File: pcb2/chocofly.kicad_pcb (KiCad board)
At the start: 2 copper layers, 341.3 x 148.9 mm, 173 parts, among them P1 battery+, P2 battery-, SW1 SW_Push, SW11 SW_Push, SW12 SW_Push, SW13 SW_Push, SW14 SW_Push, SW15 SW_Push, SW16 SW_Push, SW17 SW_Push, SW18 SW_Push, SW19 SW_Push, SW2 SW_Push, SW20 SW_Push, SW21 SW_Push, SW22 SW_Push, SW23 SW_Push, SW24 SW_Push, SW25 SW_Push, SW26 SW_Push, SW27 SW_Push, SW28 SW_Push, SW29 SW_Push, SW3 SW_Push, SW30 SW_Push, SW31 SW_Push, SW32 SW_Push, SW33 SW_Push, SW34 SW_Push, SW35 SW_Push, SW36 SW_Push, SW37 SW_Push, SW38 SW_Push, SW39 SW_Push, SW4 SW_Push, SW40 SW_Push, SW41 SW_Push, SW42 SW_Push, SW43 SW_Push, SW44 SW_Push, SW45 SW_Push, SW46 SW_Push, SW47 SW_Push, SW48 SW_Push, SW49 SW_Push, SW5 SW_Push, SW50 SW_Push, SW51 SW_Push, SW52 SW_Push, SW53 SW_Push, SW54 SW_Push, SW55 SW_Push, SW56 SW_Push, SW57 SW_Push, SW58 SW_Push, SW59 SW_Push, SW6 SW_Push, SW60 SW_Push, SW61 SW_Push, SW62 Reset, SW63 Power, SW7 SW_Push, SW8 SW_Push, SW9 SW_Push

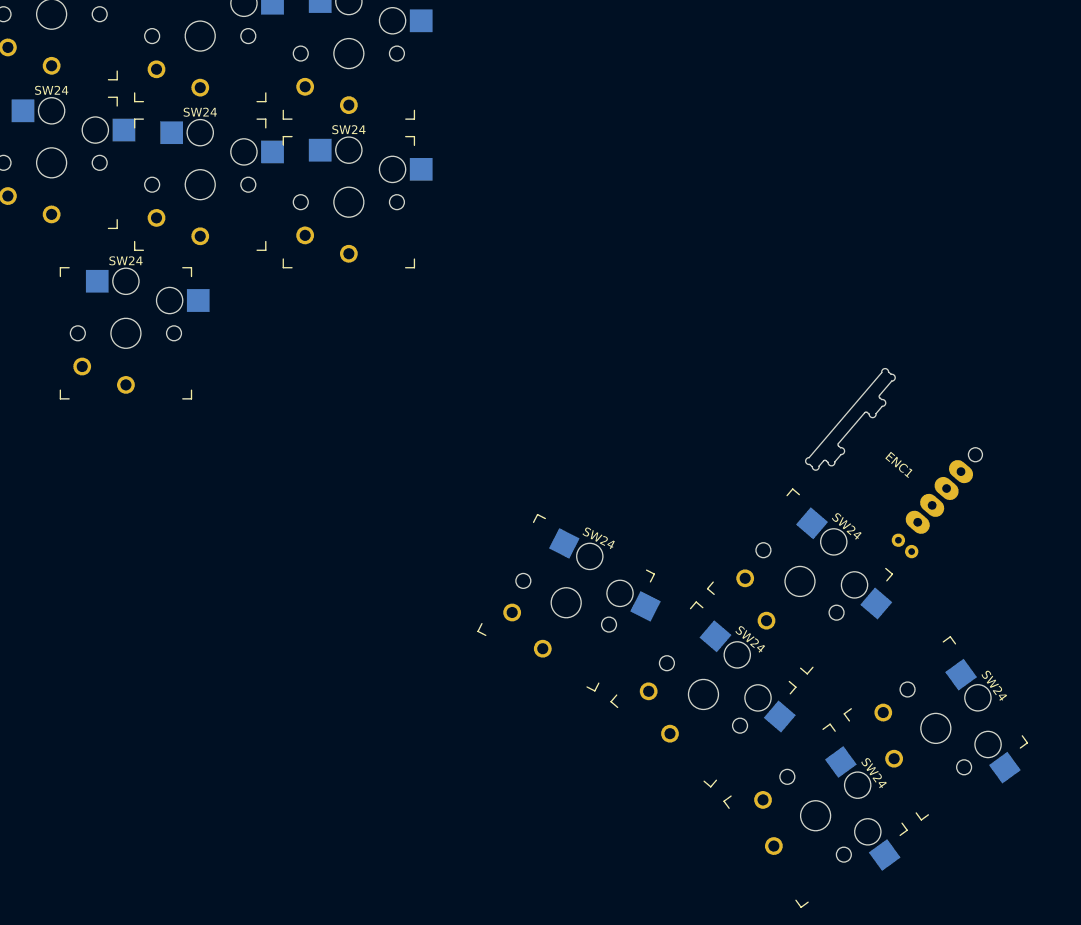
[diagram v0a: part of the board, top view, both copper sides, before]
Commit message: wip
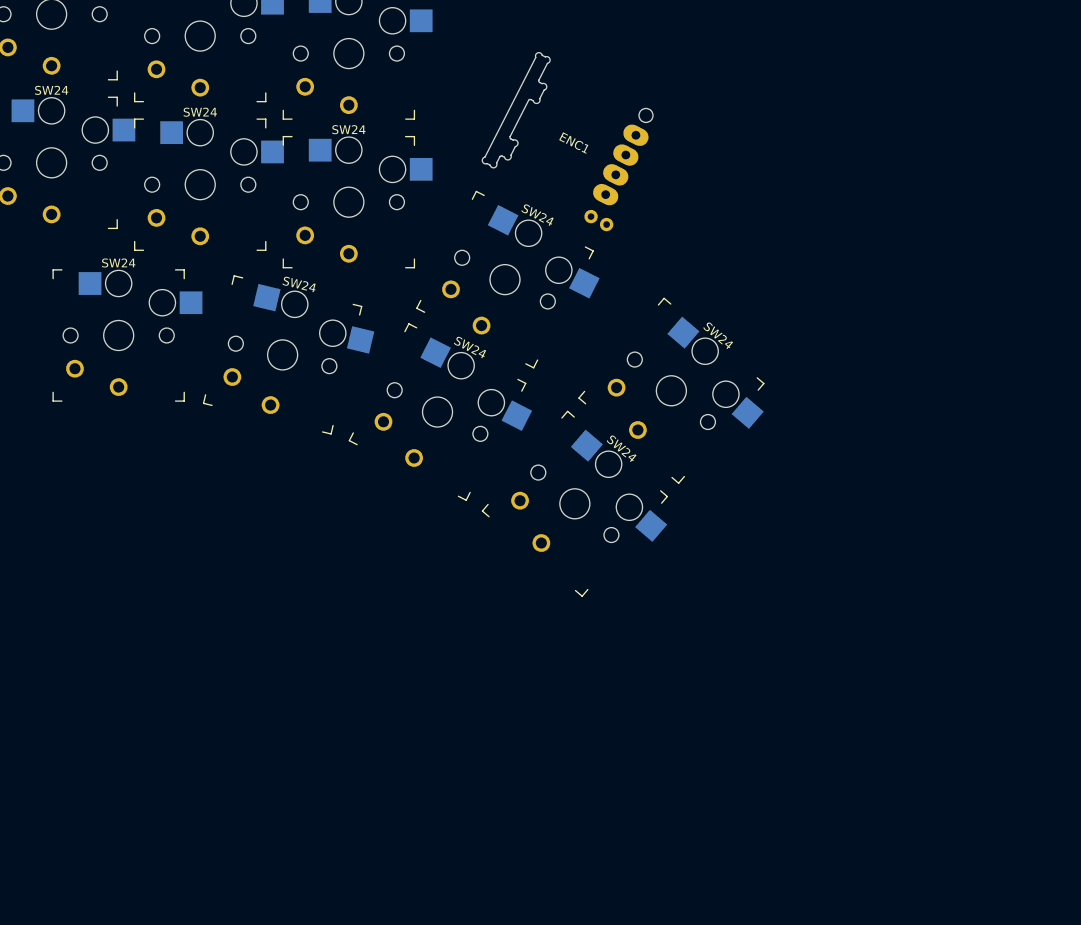
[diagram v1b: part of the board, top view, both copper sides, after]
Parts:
- removed the SW24 at (22.1, 243.2)
- removed the SW24 at (6.60, 226.4)
- removed the SW24 at (8.39, 253.2)
- removed the SW24 at (-4.44, 239.3)
- added SW24: SW_Push, footprints:Kailh_socket_PG1350_optional_chosfox, F.Cu at (-8.11, 204.6)
- added SW24: SW_Push, footprints:Kailh_socket_PG1350_optional_chosfox, F.Cu at (-27.1, 191.9)
- added SW24: SW_Push, footprints:Kailh_socket_PG1350_optional_chosfox, F.Cu at (-19.1, 217.5)
- added SW24: SW_Push, footprints:Kailh_socket_PG1350_optional_chosfox, F.Cu at (-34.9, 207.0)
- moved ENC1 52.3 mm to (-19.2, 176.3), turned to 153 degrees
- moved SW24 43.1 mm to (-52.6, 200.5), turned to 346.5 degrees
- moved SW24 0.87 mm to (-71.3, 198.2)

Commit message: General layout is ready
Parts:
- removed the ENC1 at (-19.2, 176.3)
- removed the SW24 at (-8.11, 204.6)
- removed the SW24 at (-131.4, 168.5)
- removed the SW24 at (-45.0, 166.0)
- removed the SW24 at (-62.0, 181.0)
- removed the SW24 at (-96.0, 164.0)
- removed the SW24 at (-130.3, 185.5)
- removed the SW24 at (-96.0, 181.0)
- removed the SW24 at (-114.4, 167.5)
- removed the SW24 at (-79.0, 178.5)
- removed the SW24 at (-113.4, 184.4)
- removed the SW24 at (-45.0, 183.0)
- removed the SW24 at (-27.1, 191.9)
- removed the SW24 at (-79.0, 144.5)
- removed the SW24 at (-62.0, 147.0)
- removed the SW24 at (-132.4, 151.5)
- removed the SW24 at (-45.0, 149.0)
- removed the SW24 at (-96.0, 147.0)
- removed the SW24 at (-115.4, 150.5)
- removed the SW24 at (-45.0, 132.0)
- removed the SW24 at (-62.0, 130.0)
- removed the SW24 at (-79.0, 127.5)
- removed the SW24 at (-96.0, 130.0)
- removed the SW24 at (-19.1, 217.5)
- removed the SW24 at (-116.5, 133.5)
- removed the SW24 at (-34.9, 207.0)
- removed the SW24 at (-52.6, 200.5)
- removed the SW24 at (-71.3, 198.2)
- removed the SW24 at (-133.4, 134.6)
- removed the SW24 at (-79.0, 161.5)
- removed the SW24 at (-62.0, 164.0)
- added ENC1: EVQWGD001, footprints:EVQWGD001, F.Cu at (-15.3, 219.8)
- added ENC1: EVQWGD001, footprints:EVQWGD001, F.Cu at (-53.7, 219.8)
- added SW24: SW_Push, footprints:Kailh_socket_PG1350_optional_chosfox, F.Cu at (-19.5, 249.9)
- added SW24: SW_Push, footprints:Kailh_socket_PG1350_optional_chosfox, F.Cu at (72.2, 172.3)
- added SW24: SW_Push, footprints:Kailh_socket_PG1350_optional_chosfox, F.Cu at (52.5, 173.4)
- added SW24: SW_Push, footprints:Kailh_socket_PG1350_optional_chosfox, F.Cu at (56.5, 190.0)
- added SW24: SW_Push, footprints:Kailh_socket_PG1350_optional_chosfox, F.Cu at (27.4, 214.4)
- added SW24: SW_Push, footprints:Kailh_socket_PG1350_optional_chosfox, F.Cu at (91.9, 186.1)
- added SW24: SW_Push, footprints:Kailh_socket_PG1350_optional_chosfox, F.Cu at (75.2, 189.0)
- added SW24: SW_Push, footprints:Kailh_socket_PG1350_optional_chosfox, F.Cu at (94.9, 202.8)
- added SW24: SW_Push, footprints:Kailh_socket_PG1350_optional_chosfox, F.Cu at (39.4, 191.5)
- added SW24: SW_Push, footprints:Kailh_socket_PG1350_optional_chosfox, F.Cu at (7.36, 203.8)
- added SW24: SW_Push, footprints:Kailh_socket_PG1350_optional_chosfox, F.Cu at (86.0, 152.6)
- added SW24: SW_Push, footprints:Kailh_socket_PG1350_optional_chosfox, F.Cu at (40.5, 229.0)
- added SW24: SW_Push, footprints:Kailh_socket_PG1350_optional_chosfox, F.Cu at (89.0, 169.4)
- added SW24: SW_Push, footprints:Kailh_socket_PG1350_optional_chosfox, F.Cu at (3.39, 187.3)
- added SW24: SW_Push, footprints:Kailh_socket_PG1350_optional_chosfox, F.Cu at (23.4, 197.9)
- added SW24: SW_Push, footprints:Kailh_socket_PG1350_optional_chosfox, F.Cu at (78.1, 205.8)
- added SW24: SW_Push, footprints:Kailh_socket_PG1350_optional_chosfox, F.Cu at (15.5, 164.9)
- added SW24: SW_Push, footprints:Kailh_socket_PG1350_optional_chosfox, F.Cu at (-0.58, 170.8)
- added SW24: SW_Push, footprints:Kailh_socket_PG1350_optional_chosfox, F.Cu at (48.5, 156.9)
- added SW24: SW_Push, footprints:Kailh_socket_PG1350_optional_chosfox, F.Cu at (43.3, 208.0)
- added SW24: SW_Push, footprints:Kailh_socket_PG1350_optional_chosfox, F.Cu at (35.4, 175.0)
- added SW24: SW_Push, footprints:Kailh_socket_PG1350_optional_chosfox, F.Cu at (11.3, 220.4)
- added SW24: SW_Push, footprints:Kailh_socket_PG1350_optional_chosfox, F.Cu at (69.3, 155.6)
- added SW24: SW_Push, footprints:Kailh_socket_PG1350_optional_chosfox, F.Cu at (60.5, 206.5)
- added SW24: SW_Push, footprints:Kailh_socket_PG1350_optional_chosfox, F.Cu at (-49.6, 249.9)
- added SW24: SW_Push, footprints:Kailh_socket_PG1350_optional_chosfox, F.Cu at (-65.1, 233.1)
- added SW24: SW_Push, footprints:Kailh_socket_PG1350_optional_chosfox, F.Cu at (-63.3, 259.9)
- added SW24: SW_Push, footprints:Kailh_socket_PG1350_optional_chosfox, F.Cu at (-76.1, 246.1)
- added SW24: SW_Push, footprints:Kailh_socket_PG1350_optional_chosfox, F.Cu at (-91.8, 235.6)
- added SW24: SW_Push, footprints:Kailh_socket_PG1350_optional_chosfox, F.Cu at (-109.6, 229.0)
- added SW24: SW_Push, footprints:Kailh_socket_PG1350_optional_chosfox, F.Cu at (-155.1, 152.6)
- added SW24: SW_Push, footprints:Kailh_socket_PG1350_optional_chosfox, F.Cu at (-108.4, 191.5)
- added SW24: SW_Push, footprints:Kailh_socket_PG1350_optional_chosfox, F.Cu at (-92.5, 197.9)
- added SW24: SW_Push, footprints:Kailh_socket_PG1350_optional_chosfox, F.Cu at (22.8, 235.6)
- added SW24: SW_Push, footprints:Kailh_socket_PG1350_optional_chosfox, F.Cu at (-161.0, 186.1)
- added SW24: SW_Push, footprints:Kailh_socket_PG1350_optional_chosfox, F.Cu at (-76.4, 203.8)
- added SW24: SW_Push, footprints:Kailh_socket_PG1350_optional_chosfox, F.Cu at (-96.5, 214.4)
- added SW24: SW_Push, footprints:Kailh_socket_PG1350_optional_chosfox, F.Cu at (-125.6, 190.0)
- added SW24: SW_Push, footprints:Kailh_socket_PG1350_optional_chosfox, F.Cu at (-163.9, 202.8)
- added SW24: SW_Push, footprints:Kailh_socket_PG1350_optional_chosfox, F.Cu at (-129.5, 206.5)
- added SW24: SW_Push, footprints:Kailh_socket_PG1350_optional_chosfox, F.Cu at (-144.3, 189.0)
- added SW24: SW_Push, footprints:Kailh_socket_PG1350_optional_chosfox, F.Cu at (-112.4, 208.0)
- added SW24: SW_Push, footprints:Kailh_socket_PG1350_optional_chosfox, F.Cu at (-147.2, 205.8)
- added SW24: SW_Push, footprints:Kailh_socket_PG1350_optional_chosfox, F.Cu at (-80.4, 220.4)
- added SW24: SW_Push, footprints:Kailh_socket_PG1350_optional_chosfox, F.Cu at (7.07, 246.1)
- added SW24: SW_Push, footprints:Kailh_socket_PG1350_optional_chosfox, F.Cu at (-104.5, 175.0)
- added SW24: SW_Push, footprints:Kailh_socket_PG1350_optional_chosfox, F.Cu at (-88.5, 181.4)
- added SW24: SW_Push, footprints:Kailh_socket_PG1350_optional_chosfox, F.Cu at (-158.0, 169.4)
- added SW24: SW_Push, footprints:Kailh_socket_PG1350_optional_chosfox, F.Cu at (-72.5, 187.3)
- added SW24: SW_Push, footprints:Kailh_socket_PG1350_optional_chosfox, F.Cu at (-121.6, 173.4)
- added SW24: SW_Push, footprints:Kailh_socket_PG1350_optional_chosfox, F.Cu at (-141.3, 172.3)
- added SW24: SW_Push, footprints:Kailh_socket_PG1350_optional_chosfox, F.Cu at (-68.5, 170.8)
- added SW24: SW_Push, footprints:Kailh_socket_PG1350_optional_chosfox, F.Cu at (-84.6, 164.8)
- added SW24: SW_Push, footprints:Kailh_socket_PG1350_optional_chosfox, F.Cu at (-100.5, 158.4)
- added SW24: SW_Push, footprints:Kailh_socket_PG1350_optional_chosfox, F.Cu at (-117.6, 156.9)
- added SW24: SW_Push, footprints:Kailh_socket_PG1350_optional_chosfox, F.Cu at (-3.97, 233.1)
- added SW24: SW_Push, footprints:Kailh_socket_PG1350_optional_chosfox, F.Cu at (-138.3, 155.6)
- added SW24: SW_Push, footprints:Kailh_socket_PG1350_optional_chosfox, F.Cu at (31.4, 158.5)
- added SW24: SW_Push, footprints:Kailh_socket_PG1350_optional_chosfox, F.Cu at (-5.75, 259.9)
- added SW24: SW_Push, footprints:Kailh_socket_PG1350_optional_chosfox, F.Cu at (19.5, 181.4)
